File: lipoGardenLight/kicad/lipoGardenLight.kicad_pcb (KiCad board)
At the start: 2 copper layers, 52.8 x 31.1 mm, 14 parts, among them Q1 BC557, Q2 SS8050, Q3 SS8050

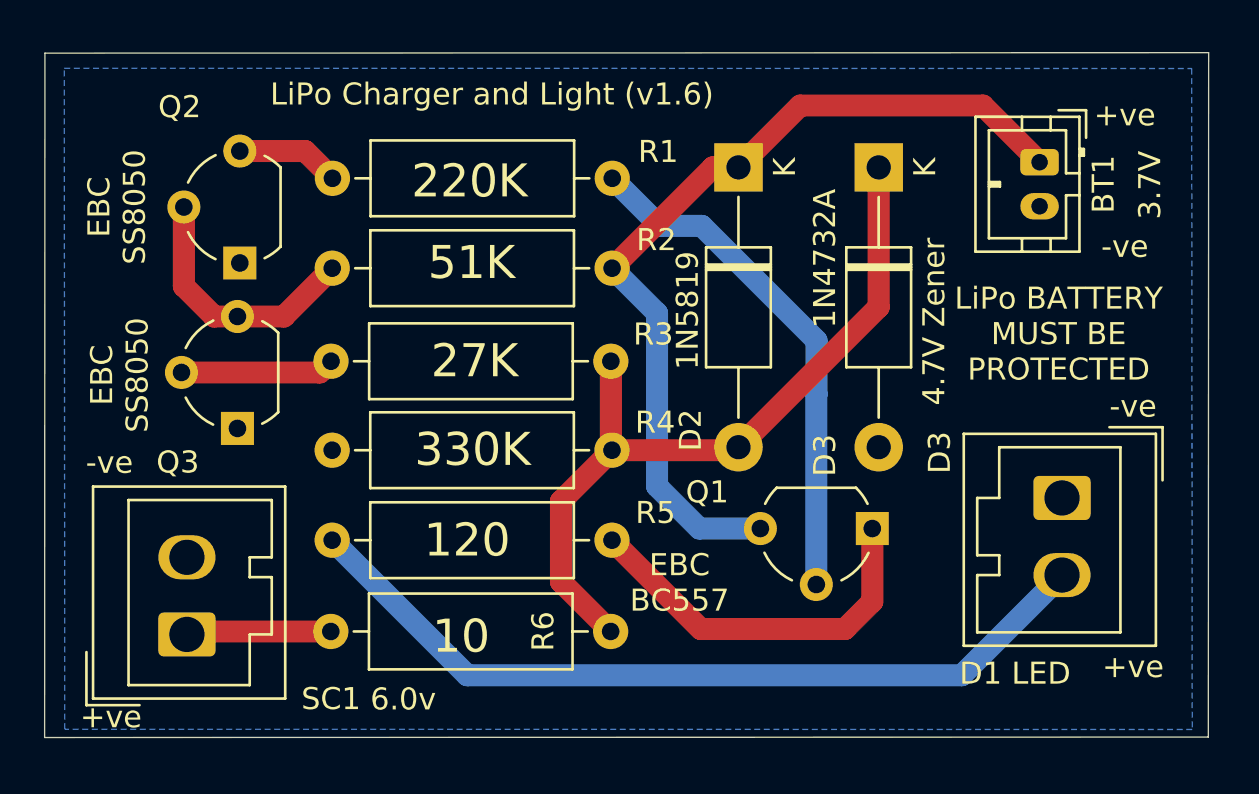
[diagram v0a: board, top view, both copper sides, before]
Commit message: Update PCB's
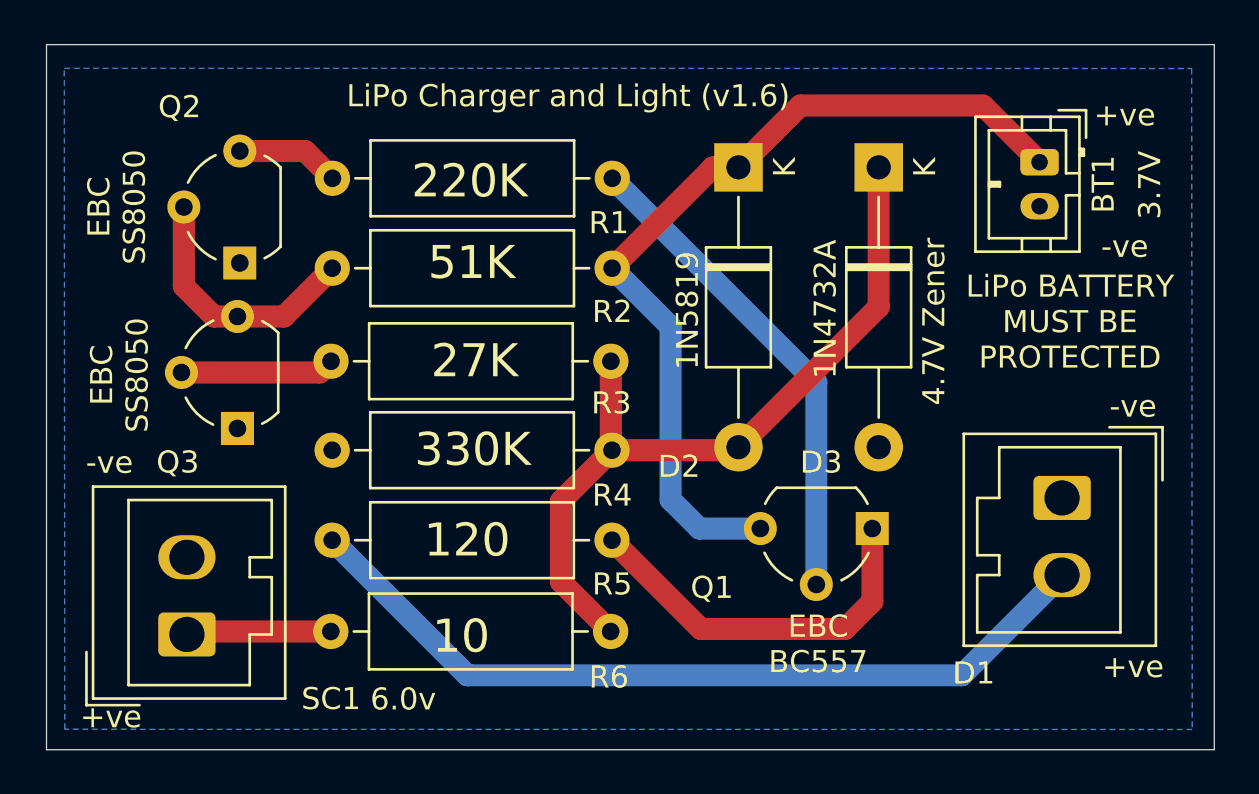
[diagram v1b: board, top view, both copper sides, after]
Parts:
- D1: renamed from D1 LED
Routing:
- net Net-(Q1-B): track 23.4 -> 22.3 mm
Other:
- board size 52.8 x 31.1 mm -> 53 x 32 mm
- board text removed: "D3"
